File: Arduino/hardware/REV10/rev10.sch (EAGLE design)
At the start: 46 parts, among them IC2 ATMEGA168-AU, Q1 32768Hz, U1 TC1185SMD, U2 ARDUINO

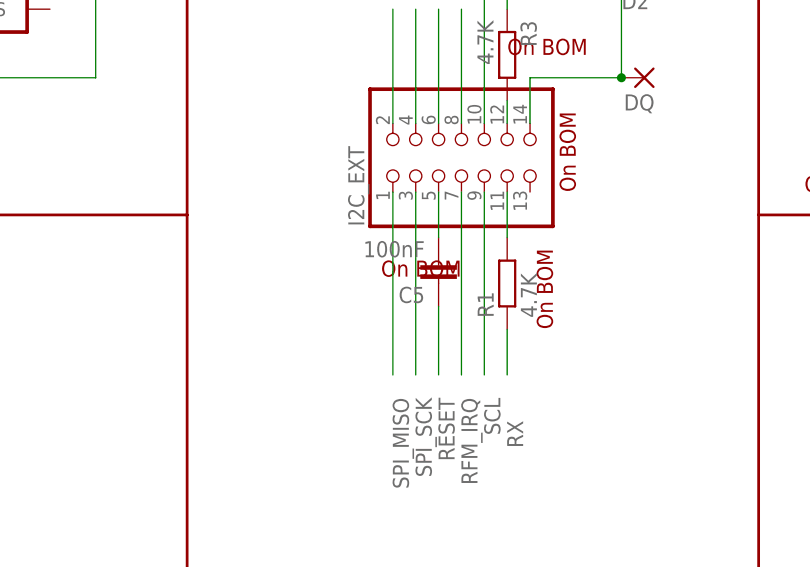
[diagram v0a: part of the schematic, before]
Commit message: rev 10 with 5 tracks left
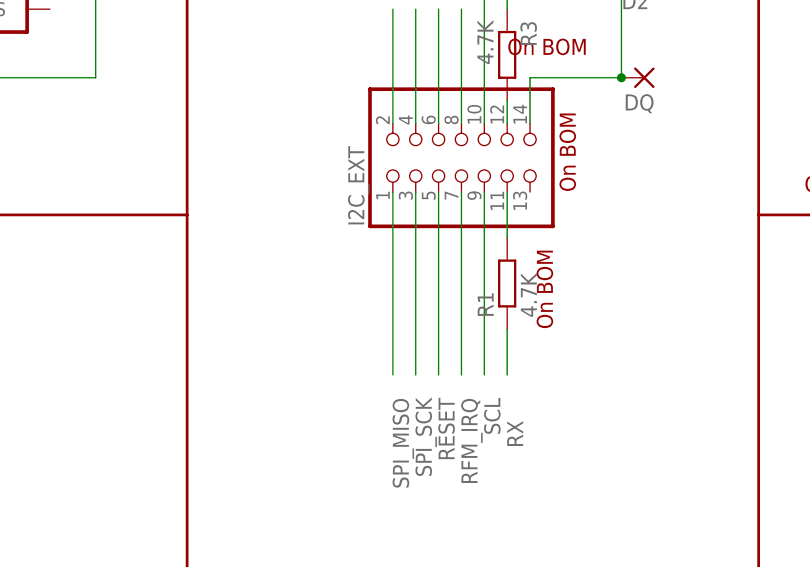
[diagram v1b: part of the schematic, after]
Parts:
- removed C5: 100nF, resistor:C-EUC0603
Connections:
- removed net N$25: C5.2, I2C_EXT.5
- net RESET: now also I2C_EXT.5; no longer C5.1
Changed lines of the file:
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@@
 <part name="R1" library="resistor" deviceset="R-EU_" device="R0603" value="4.7K"/>
 <part name="R3" library="resistor" deviceset="R-EU_" device="R0603" value="4.7K"/>
-<part name="C5" library="resistor" deviceset="C-EU" device="C0603" value="100nF"/>
 <part name="I2C_EXT" library="pinhead" deviceset="PINHD-2X7" device=""/>
 <part name="IC2" library="Arduino-AVR" deviceset="ATMEGA168" device="-AU"/>
@@
 <text x="17.78" y="139.7" size="1.778" layer="94">On BOM</text>
 <text x="134.62" y="195.58" size="1.778" layer="94" rot="R90">On BOM</text>
-<text x="124.46" y="203.2" size="1.778" layer="94" rot="R180">On BOM</text>
 <text x="129.54" y="226.06" size="1.778" layer="94">On BOM</text>
 <text x="205.74" y="231.14" size="1.778" layer="94" rot="R90">On BOM</text>
@@
 <instance part="R1" gate="G$1" x="129.54" y="200.66" rot="R90"/>
 <instance part="R3" gate="G$1" x="129.54" y="226.06" rot="R270"/>
-<instance part="C5" gate="G$1" x="121.92" y="200.66" rot="R180"/>
 <instance part="I2C_EXT" gate="A" x="124.46" y="213.36" rot="R90"/>
 <instance part="IC2" gate="1" x="195.58" y="91.44"/>
@@
 </segment>
 <segment>
-<pinref part="C5" gate="G$1" pin="1"/>
-<wire x1="121.92" y1="198.12" x2="121.92" y2="190.5" width="0.1524" layer="91"/>
 <label x="121.92" y="187.96" size="1.778" layer="95" rot="R270"/>
+<pinref part="I2C_EXT" gate="A" pin="5"/>
+<wire x1="121.92" y1="190.5" x2="121.92" y2="210.82" width="0.1524" layer="91"/>
 </segment>
 <segment>
@@
 </segment>
 </net>
-<net name="N$25" class="0">
-<segment>
-<wire x1="121.92" y1="210.82" x2="121.92" y2="205.74" width="0.1524" layer="91"/>
-<pinref part="C5" gate="G$1" pin="2"/>
-<pinref part="I2C_EXT" gate="A" pin="5"/>
-</segment>
-</net>
